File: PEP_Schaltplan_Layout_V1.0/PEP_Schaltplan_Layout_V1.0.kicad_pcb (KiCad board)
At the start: 2 copper layers, 117.5 x 83 mm, 120 parts, among them Q3 BC546, Q4 BC556, Q5 BF256, SW1 SW_DIP_x04, SW10 SW_DIP_x04, SW11 SW_DIP_x04, SW12 SW_DIP_x04, SW13 SW_DIP_x04, SW14 SW_DIP_x04, SW2 SW_DIP_x04, SW3 SW_DIP_x04, SW4 SW_DIP_x04, SW5 SW_DIP_x04, SW6 SW_DIP_x04, SW7 SW_DIP_x04, SW8 SW_DIP_x04, SW9 SW_DIP_x04, U12 AD822ANZ_new, U13 LT1819, U14 LT1819, U15 LT1819, U16 LT1819, U23 LM7905_TO220, U24 LM7805_TO220

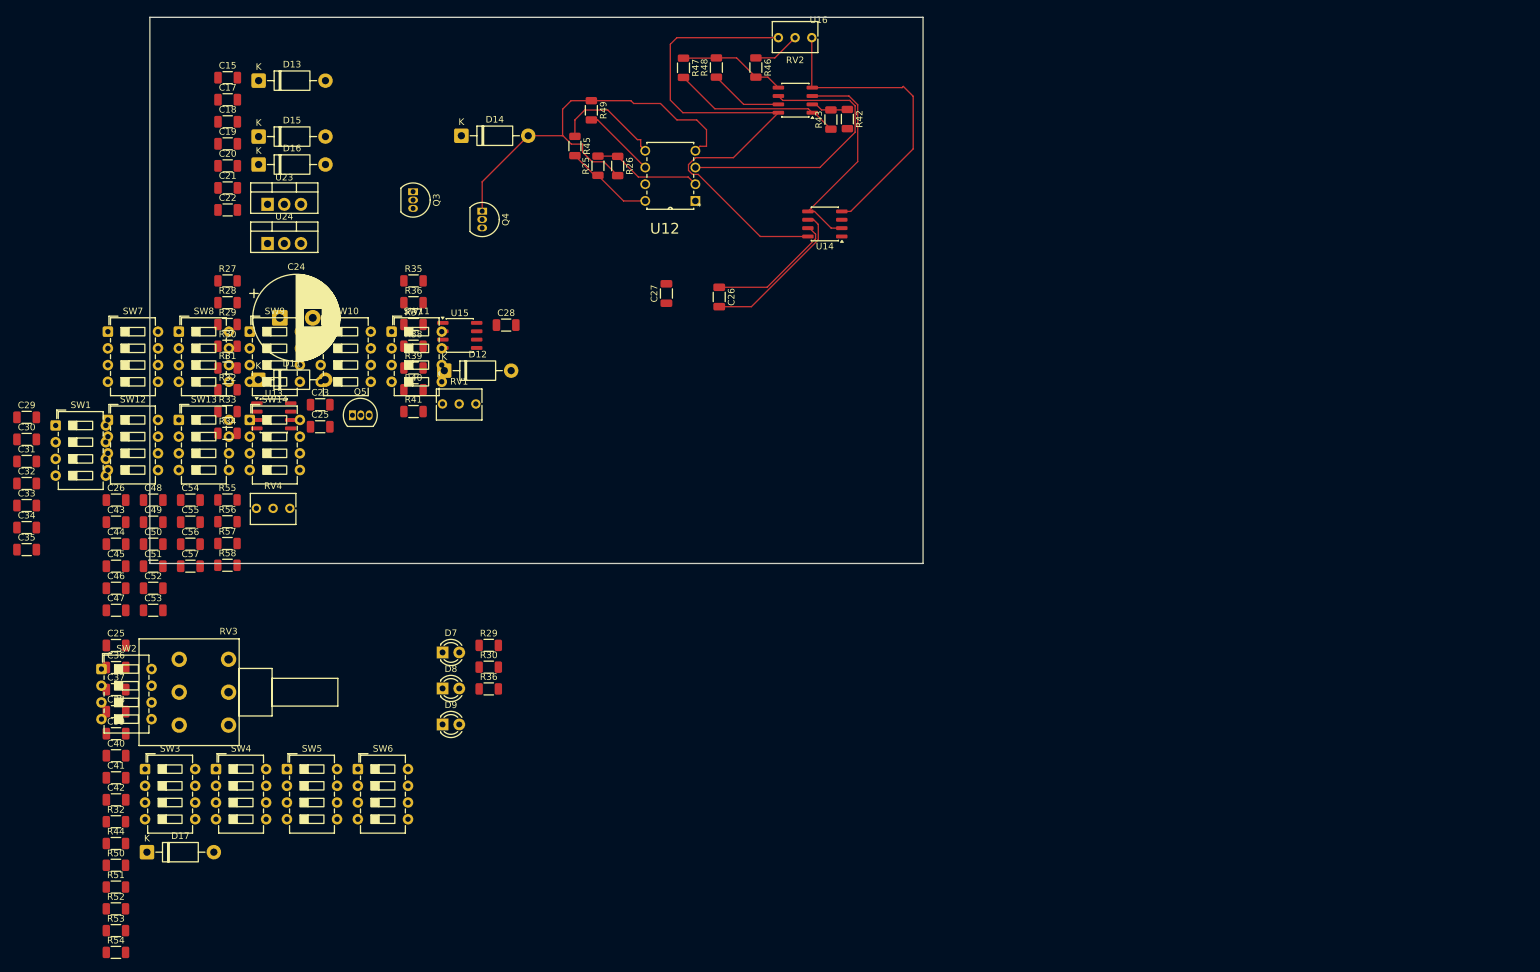
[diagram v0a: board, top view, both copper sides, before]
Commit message: Überarbeitung und Bereinigung
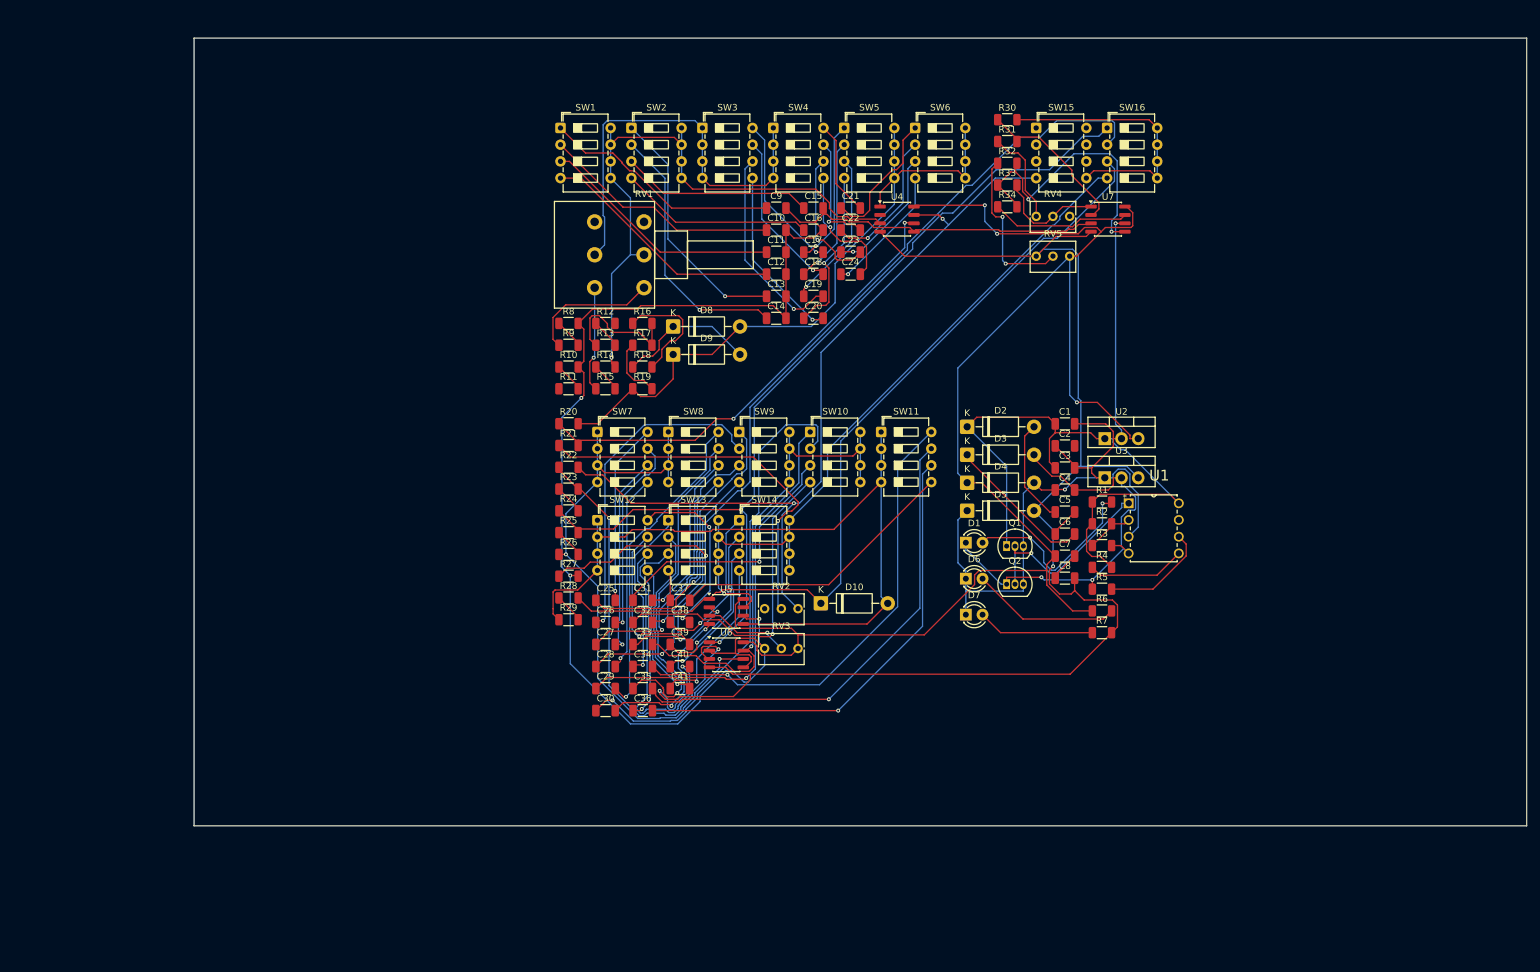
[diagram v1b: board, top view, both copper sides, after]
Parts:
- removed the C25 at (67.9, 99.7)
- removed the C25 at (36.9, 133.0)
- removed the C26 at (128.5, 80.0)
- removed the C26 at (36.9, 110.9)
- removed C42: 6.8n, Capacitor_SMD:C_1206_3216Metric
- removed C43, C50: 4.7n, Capacitor_SMD:C_1206_3216Metric
- removed C44: 470p, Capacitor_SMD:C_1206_3216Metric
- removed C45: 100p, Capacitor_SMD:C_1206_3216Metric
- removed C46, C53, C54: 47p, Capacitor_SMD:C_1206_3216Metric
- removed C47, C55: 22p, Capacitor_SMD:C_1206_3216Metric
- removed C48, C49, C56, C57: 0, Capacitor_SMD:C_1206_3216Metric
- removed C51: 1n, Capacitor_SMD:C_1206_3216Metric
- removed C52: 220p, Capacitor_SMD:C_1206_3216Metric
- removed D11, D12, D17: 1N4148, Diode_THT:D_DO-41_SOD81_P10.16mm_Horizontal
- removed D13, D14, D15, D16: 1N4002, Diode_THT:D_DO-41_SOD81_P10.16mm_Horizontal
- removed Q3: BC546, Package_TO_SOT_THT:TO-92_Inline
- removed Q4: BC556, Package_TO_SOT_THT:TO-92_Inline
- removed Q5: BF256, Package_TO_SOT_THT:TO-92L_Inline
- removed the R29 at (93.5, 132.9)
- removed the R29 at (53.8, 84.2)
- removed the R30 at (93.5, 136.3)
- removed the R30 at (53.8, 87.5)
- removed the R32 at (53.8, 94.1)
- removed the R32 at (36.8, 159.7)
- removed R35, R55: 1k, Resistor_SMD:R_1206_3216Metric
- removed R36: 2k2, Resistor_SMD:R_1206_3216Metric
- removed R36: 20k, Resistor_SMD:R_1206_3216Metric
- removed R37, R44, R46, R47, R48: 10k, Resistor_SMD:R_1206_3216Metric
- removed R38: 190k, Resistor_SMD:R_1206_3216Metric
- removed R39: 18k, Resistor_SMD:R_1206_3216Metric
- removed R40: 100k, Resistor_SMD:R_1206_3216Metric
- removed R41: 12k, Resistor_SMD:R_1206_3216Metric
- removed R42, R43: 5k, Resistor_SMD:R_1206_3216Metric
- removed R45, R49: R, Resistor_SMD:R_1206_3216Metric
- removed R50, R51, R52, R53, R54, R57, R58: 0, Resistor_SMD:R_1206_3216Metric
- removed R56: ^0, Resistor_SMD:R_1206_3216Metric
- removed U12: AD822ANZ_new, KiCad Footprint Bib:DIP8
- removed U13, U14, U15, U16: LT1819, Package_SO:SO-8_3.9x4.9mm_P1.27mm
- removed U23: LM7905_TO220, Package_TO_SOT_THT:TO-220-3_Vertical
- removed U24: LM7805_TO220, Package_TO_SOT_THT:TO-220-3_Vertical
- added C1: 1µ, Capacitor_SMD:C_1206_3216Metric, F.Cu at (181.1, 99.3)
- added C10: 6.8n, Capacitor_SMD:C_1206_3216Metric, F.Cu at (137.2, 69.8)
- added C11: 6.8n, Capacitor_SMD:C_1206_3216Metric, F.Cu at (137.2, 73.2)
- added C12: 6.8n, Capacitor_SMD:C_1206_3216Metric, F.Cu at (137.2, 76.5)
- added C13: 6.8n, Capacitor_SMD:C_1206_3216Metric, F.Cu at (137.2, 79.9)
- added C14: 6.8n, Capacitor_SMD:C_1206_3216Metric, F.Cu at (137.2, 83.2)
- added C16: 6.8n, Capacitor_SMD:C_1206_3216Metric, F.Cu at (142.8, 69.8)
- added C2: 1µ, Capacitor_SMD:C_1206_3216Metric, F.Cu at (181.1, 102.6)
- added C25: 22n, Capacitor_SMD:C_1206_3216Metric, F.Cu at (111.3, 126.1)
- added C26: 4.7n, Capacitor_SMD:C_1206_3216Metric, F.Cu at (111.3, 129.5)
- added C3: 100n, Capacitor_SMD:C_1206_3216Metric, F.Cu at (181.1, 106.0)
- added C4: 100n, Capacitor_SMD:C_1206_3216Metric, F.Cu at (181.1, 109.3)
- added C5: 1µ, Capacitor_SMD:C_1206_3216Metric, F.Cu at (181.1, 112.7)
- added C6: 1µ, Capacitor_SMD:C_1206_3216Metric, F.Cu at (181.1, 116.0)
- added C7: 100n, Capacitor_SMD:C_1206_3216Metric, F.Cu at (181.1, 119.4)
- added C8: 100n, Capacitor_SMD:C_1206_3216Metric, F.Cu at (181.1, 122.7)
- added C9: 6.8n, Capacitor_SMD:C_1206_3216Metric, F.Cu at (137.2, 66.5)
- added D1: LED, LED_THT:LED_D3.0mm, F.Cu at (166.0, 117.3)
- added D10: 1N4148, Diode_THT:D_DO-41_SOD81_P10.16mm_Horizontal, F.Cu at (144.0, 126.6)
- added D2: 1N4002, Diode_THT:D_DO-41_SOD81_P10.16mm_Horizontal, F.Cu at (166.2, 99.7)
- added D3: 1N4002, Diode_THT:D_DO-41_SOD81_P10.16mm_Horizontal, F.Cu at (166.2, 104.0)
- added D4: 1N4002, Diode_THT:D_DO-41_SOD81_P10.16mm_Horizontal, F.Cu at (166.2, 108.2)
- added D5: 1N4002, Diode_THT:D_DO-41_SOD81_P10.16mm_Horizontal, F.Cu at (166.2, 112.5)
- added D6: LED, LED_THT:LED_D3.0mm, F.Cu at (166.0, 122.8)
- added Q1: BC546, Package_TO_SOT_THT:TO-92_Inline, F.Cu at (172.2, 117.9)
- added Q2: BC556, Package_TO_SOT_THT:TO-92_Inline, F.Cu at (172.2, 123.7)
- added R1: 2k2, Resistor_SMD:R_1206_3216Metric, F.Cu at (186.7, 111.2)
- added R10: 0, Resistor_SMD:R_1206_3216Metric, F.Cu at (105.6, 90.6)
- added R11: 10k, Resistor_SMD:R_1206_3216Metric, F.Cu at (105.6, 94.0)
- added R12: 0, Resistor_SMD:R_1206_3216Metric, F.Cu at (111.2, 84.0)
- added R13: 10k, Resistor_SMD:R_1206_3216Metric, F.Cu at (111.2, 87.3)
- added R14: 500, Resistor_SMD:R_1206_3216Metric, F.Cu at (111.2, 90.6)
- added R15: 0, Resistor_SMD:R_1206_3216Metric, F.Cu at (111.2, 94.0)
- added R16: 24K, Resistor_SMD:R_1206_3216Metric, F.Cu at (116.8, 84.0)
- added R17: 12k, Resistor_SMD:R_1206_3216Metric, F.Cu at (116.8, 87.3)
- added R18: 0, Resistor_SMD:R_1206_3216Metric, F.Cu at (116.8, 90.6)
- added R19: 0, Resistor_SMD:R_1206_3216Metric, F.Cu at (116.8, 94.0)
- added R2: 47k, Resistor_SMD:R_1206_3216Metric, F.Cu at (186.7, 114.5)
- added R20: 1k, Resistor_SMD:R_1206_3216Metric, F.Cu at (105.6, 99.3)
- added R21: 1k, Resistor_SMD:R_1206_3216Metric, F.Cu at (105.6, 102.6)
- added R22: 10k, Resistor_SMD:R_1206_3216Metric, F.Cu at (105.6, 105.9)
- added R23: 190k, Resistor_SMD:R_1206_3216Metric, F.Cu at (105.6, 109.2)
- added R24: 0, Resistor_SMD:R_1206_3216Metric, F.Cu at (105.6, 112.5)
- added R29: ^0, Resistor_SMD:R_1206_3216Metric, F.Cu at (105.6, 129.1)
- added R3: 47k, Resistor_SMD:R_1206_3216Metric, F.Cu at (186.7, 117.8)
- added R30: 1k, Resistor_SMD:R_1206_3216Metric, F.Cu at (172.3, 53.1)
- added R32: 10k, Resistor_SMD:R_1206_3216Metric, F.Cu at (172.3, 59.7)
- added R4: R, Resistor_SMD:R_1206_3216Metric, F.Cu at (186.7, 121.1)
- added R5: R, Resistor_SMD:R_1206_3216Metric, F.Cu at (186.7, 124.4)
- added R6: 470, Resistor_SMD:R_1206_3216Metric, F.Cu at (186.7, 127.7)
- added R7: 470, Resistor_SMD:R_1206_3216Metric, F.Cu at (186.7, 131.0)
- added R8: 500, Resistor_SMD:R_1206_3216Metric, F.Cu at (105.6, 84.0)
- added R9: 0, Resistor_SMD:R_1206_3216Metric, F.Cu at (105.6, 87.3)
- added RV5: 10k, Potentiometer_THT:Potentiometer_Bourns_3266Y_Vertical, F.Cu at (181.8, 73.8)
- added SW15: SW_DIP_x04, Button_Switch_THT:SW_DIP_SPSTx04_Slide_6.7x11.72mm_W7.62mm_P2.54mm_LowProfile, F.Cu at (176.7, 54.3)
- added SW16: SW_DIP_x04, Button_Switch_THT:SW_DIP_SPSTx04_Slide_6.7x11.72mm_W7.62mm_P2.54mm_LowProfile, F.Cu at (187.5, 54.3)
- added U1: AD822ANZ_new, KiCad Footprint Bib:DIP8, F.Cu at (198.4, 119.0)
- added U2: LM7805_TO220, Package_TO_SOT_THT:TO-220-3_Vertical, F.Cu at (187.1, 101.5)
- added U3: LM7905_TO220, Package_TO_SOT_THT:TO-220-3_Vertical, F.Cu at (187.1, 107.5)
- added U4: LT1819, Package_SO:SO-8_3.9x4.9mm_P1.27mm, F.Cu at (155.5, 68.2)
- added U5: LT1819, Package_SO:SO-8_3.9x4.9mm_P1.27mm, F.Cu at (129.6, 127.8)
- added U6: LT1819, Package_SO:SO-8_3.9x4.9mm_P1.27mm, F.Cu at (129.6, 134.4)
- added U7: LT1819, Package_SO:SO-8_3.9x4.9mm_P1.27mm, F.Cu at (187.6, 68.2)
- C15, C19, C20: value 1µ -> 6.8n
- C17, C18, C21, C22: value 100n -> 6.8n
- C24: value 100µ -> 6.8n; footprint Capacitor_THT:CP_Radial_D13.0mm_P5.00mm -> Capacitor_SMD:C_1206_3216Metric
- C27: value 1µ -> 470p
- C28: value 4.7n -> 100p
- C29, C37, C38: value 6.8n -> 47p
- C30, C39: value 6.8n -> 22p
- C31, C32, C40, C41: value 6.8n -> 0
- C33: value 6.8n -> 1µ
- C34: value 6.8n -> 4.7n
- C35: value 6.8n -> 1n
- C36: value 6.8n -> 220p
- D8, D9: value LED -> 1N4148; footprint LED_THT:LED_D3.0mm -> Diode_THT:D_DO-41_SOD81_P10.16mm_Horizontal
- R25: value 47k -> 0
- R26: value 47k -> 18k
- R27: value 500 -> 100k
- R28: value 10k -> 12k
- R31: value 500 -> 1k
- R33: value 24K -> 10k
- R34: value 12k -> 10k
- RV1: value R_Potentiometer -> R_Potentiometer_Dual_Separate; footprint Potentiometer_THT:Potentiometer_Bourns_3266Y_Vertical -> Potentiometer_THT:Potentiometer_Piher_T-16H_Double_Horizontal
- RV2, RV4: value R_Potentiometer -> 10k
- RV3: value R_Potentiometer_Dual_Separate -> 10k; footprint Potentiometer_THT:Potentiometer_Piher_T-16H_Double_Horizontal -> Potentiometer_THT:Potentiometer_Bourns_3266Y_Vertical
- moved SW3 129.1 mm to (126.0, 54.3)
- moved SW4 129.1 mm to (136.7, 54.3)
- moved SW5 129.1 mm to (147.5, 54.3)
- moved SW6 129.1 mm to (158.3, 54.3)
- moved RV4 126.5 mm to (181.8, 67.8)
- moved R31 123.4 mm to (172.3, 56.4)
- moved R33 123.4 mm to (172.3, 63.0)
- moved R34 123.4 mm to (172.3, 66.3)
- moved SW2 115.1 mm to (115.2, 54.3)
- moved C29 97.2 mm to (111.3, 139.5)
- moved C30 97.2 mm to (111.3, 142.9)
- moved C31 96.0 mm to (116.9, 126.1)
- moved C33 96.0 mm to (116.9, 132.8)
- moved C34 96.0 mm to (116.9, 136.2)
- moved C35 96.0 mm to (116.9, 139.5)
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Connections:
- C15 pad 1: +7.5V -> Net-(C15-Pad1)
- C15 pad 2: GND -> 0
- C17 pad 1: +7.5V -> Net-(C17-Pad1)
- C17 pad 2: GND -> Net-(C17-Pad2)
- C18 pad 1: GND -> Net-(C18-Pad1)
- C18 pad 2: unconnected-(C18-Pad2) -> Net-(C18-Pad2)
- C19 pad 1: Net-(D13-A) -> Net-(C19-Pad1)
- C20 pad 1: Net-(C19-Pad2) -> Net-(C20-Pad1)
- C20 pad 2: Net-(D14-K) -> Net-(C20-Pad2)
- C21 pad 1: +5V -> Net-(C21-Pad1)
- C22 pad 1: Net-(C21-Pad2) -> Net-(C22-Pad1)
- C22 pad 2: -5V -> Net-(C22-Pad2)
- C23 pad 2: 0 -> Net-(C23-Pad2)
- C24 pad 1: Net-(D11-+) -> Net-(C24-Pad1)
- C24 pad 2: 0 -> Net-(C24-Pad2)
- C27 pad 1: Dreieck -> Net-(C27-Pad1)
- C28 pad 1: Sägezahn -> Net-(C28-Pad1)
- C28 pad 2: Net-(D12--) -> Net-(C28-Pad2)
- C29 pad 2: 0 -> Net-(C29-Pad2)
- C30 pad 2: 0 -> Net-(C30-Pad2)
- C31 pad 2: 0 -> Net-(C31-Pad2)
- C32 pad 2: 0 -> Net-(C32-Pad2)
- C33 pad 1: Net-(C33-Pad1) -> Dreieck
- C33 pad 2: 0 -> Net-(C33-Pad2)
- C34 pad 2: 0 -> Net-(C34-Pad2)
- C35 pad 2: 0 -> Net-(C35-Pad2)
- D8 pad 1: GND -> Net-(D8-+)
- D8 pad 2: Net-(D8-A) -> Sinus_Wien
- D9 pad 1: -7.5V -> Sinus_Wien
- D9 pad 2: Net-(D9-A) -> Net-(D8-+)
- R25 pad 1: +7.5V -> Net-(R25-Pad1)
- R25 pad 2: Net-(U12A--) -> Rechteck
- R26 pad 1: Net-(U12A--) -> Net-(U6B--)
- R26 pad 2: -7.5V -> Net-(R25-Pad1)
- R27 pad 1: Net-(R27-Pad1) -> Dreieck
- R28 pad 2: Net-(R28-Pad2) -> PWM
- R31 pad 2: Net-(U13A-+) -> Net-(U7A--)
- R33 pad 1: Net-(R33-Pad1) -> Net-(U7B-+)
- R34 pad 1: Net-(R34-Pad1) -> offset
- R34 pad 2: Net-(R33-Pad2) -> Net-(U7B-+)
- RV1 pad 1: +5v -> Net-(R9-Pad1)
- RV1 pad 2: Net-(U15A-+) -> Net-(U4A-+)
- RV1 pad 3: 0 -> unconnected-(RV1-Pad3)
- RV2 pad 1: +5v -> Sinus
- RV2 pad 3: -5v -> unconnected-(RV2-Pad3)
- RV3 pad 1: Net-(R50-Pad1) -> +5V
- RV3 pad 2: Net-(U13A-+) -> Net-(U5A-+)
- RV3 pad 3: unconnected-(RV3-Pad3) -> 0
- RV4 pad 1: Sinus -> unconnected-(RV4-Pad1)
- RV4 pad 2: Net-(R55-Pad1) -> Net-(R33-Pad2)
- RV4 pad 3: unconnected-(RV4-Pad3) -> Net-(R31-Pad1)
- SW1 pad 1: Net-(C23-Pad1) -> Net-(C9-Pad1)
- SW1 pad 2: Net-(C29-Pad1) -> Net-(C10-Pad1)
- SW1 pad 3: Net-(C30-Pad1) -> Net-(C11-Pad1)
- SW1 pad 4: Net-(C31-Pad1) -> Net-(C12-Pad1)
- SW1 pad 5: Net-(U13A-+) -> Net-(U4A-+)
- SW1 pad 6: Net-(U13A-+) -> Net-(U4A-+)
- SW1 pad 7: Net-(U13A-+) -> Net-(U4A-+)
- SW1 pad 8: Net-(U13A-+) -> Net-(U4A-+)
- SW10 pad 1: Net-(C46-Pad1) -> Net-(C29-Pad1)
- SW10 pad 2: Net-(C47-Pad1) -> Net-(C30-Pad1)
- SW10 pad 3: Net-(C48-Pad1) -> Net-(C31-Pad1)
- SW10 pad 4: Net-(C49-Pad1) -> Net-(C32-Pad1)
- SW10 pad 5: Net-(C27-Pad2) -> Net-(C33-Pad2)
- SW10 pad 6: Net-(C27-Pad2) -> Net-(C33-Pad2)
- SW10 pad 7: Net-(C27-Pad2) -> Net-(C33-Pad2)
- SW10 pad 8: Net-(C27-Pad2) -> Net-(C33-Pad2)
- SW11 pad 1: Net-(D12--) -> Net-(D10--)
- SW11 pad 2: Net-(D12--) -> Net-(D10--)
- SW11 pad 3: Net-(D12--) -> Net-(D10--)
- SW11 pad 4: Net-(D12--) -> Net-(D10--)
- SW11 pad 5: Net-(C53-Pad2) -> Net-(C37-Pad2)
- SW11 pad 6: Net-(C52-Pad2) -> Net-(C36-Pad2)
- SW11 pad 7: Net-(C51-Pad2) -> Net-(C35-Pad2)
- SW11 pad 8: Net-(C50-Pad2) -> Net-(C34-Pad2)
- SW12 pad 1: Net-(D12--) -> Net-(D10--)
- SW12 pad 2: Net-(D12--) -> Net-(D10--)
- SW12 pad 3: Net-(D12--) -> Net-(D10--)
- SW12 pad 4: Net-(D12--) -> Net-(D10--)
- SW12 pad 5: Net-(C57-Pad2) -> Net-(C41-Pad2)
- SW12 pad 6: Net-(C56-Pad2) -> Net-(C40-Pad2)
- SW12 pad 7: Net-(C55-Pad2) -> Net-(C39-Pad2)
- SW12 pad 8: Net-(C54-Pad2) -> Net-(C38-Pad2)
- SW13 pad 1: Net-(C50-Pad1) -> Net-(C34-Pad1)
- SW13 pad 2: Net-(C51-Pad1) -> Net-(C35-Pad1)
- SW13 pad 3: Net-(C52-Pad1) -> Net-(C36-Pad1)
- SW13 pad 4: Net-(C53-Pad1) -> Net-(C37-Pad1)
- SW14 pad 1: Net-(C54-Pad1) -> Net-(C38-Pad1)
- SW14 pad 2: Net-(C55-Pad1) -> Net-(C39-Pad1)
- SW14 pad 3: Net-(C56-Pad1) -> Net-(C40-Pad1)
- SW14 pad 4: Net-(C57-Pad1) -> Net-(C41-Pad1)
- SW2 pad 1: Net-(C32-Pad1) -> Net-(C13-Pad1)
- SW2 pad 2: Net-(C33-Pad1) -> Net-(C14-Pad1)
- SW2 pad 3: Net-(C34-Pad1) -> Net-(C15-Pad1)
- SW2 pad 4: Net-(C35-Pad1) -> Net-(C16-Pad1)
- SW2 pad 5: Net-(U13A-+) -> Net-(U4A-+)
- SW2 pad 6: Net-(U13A-+) -> Net-(U4A-+)
- SW2 pad 7: Net-(U13A-+) -> Net-(U4A-+)
- SW2 pad 8: Net-(U13A-+) -> Net-(U4A-+)
- SW3 pad 1: Net-(C25-Pad1) (its old number) -> Net-(RV1-Pad5)
- SW3 pad 2: Net-(C36-Pad1) -> Net-(RV1-Pad5)
- SW3 pad 3: Net-(C37-Pad1) -> Net-(RV1-Pad5)
- SW3 pad 4: Net-(C38-Pad1) -> Net-(RV1-Pad5)
- SW3 pad 5: /Wien-Robinson-Generator/Sinus -> Net-(C20-Pad2)
- SW3 pad 6: /Wien-Robinson-Generator/Sinus -> Net-(C19-Pad2)
- SW3 pad 7: /Wien-Robinson-Generator/Sinus -> Net-(C18-Pad2)
- SW3 pad 8: /Wien-Robinson-Generator/Sinus -> Net-(C17-Pad2)
- SW4 pad 1: Net-(C39-Pad1) -> Net-(RV1-Pad5)
- SW4 pad 2: Net-(C40-Pad1) -> Net-(RV1-Pad5)
- SW4 pad 3: Net-(C41-Pad1) -> Net-(RV1-Pad5)
- SW4 pad 4: Net-(C42-Pad1) -> Net-(RV1-Pad5)
- SW4 pad 5: /Wien-Robinson-Generator/Sinus -> Net-(C24-Pad2)
- SW4 pad 6: /Wien-Robinson-Generator/Sinus -> Net-(C23-Pad2)
- SW4 pad 7: /Wien-Robinson-Generator/Sinus -> Net-(C22-Pad2)
- SW4 pad 8: /Wien-Robinson-Generator/Sinus -> Net-(C21-Pad2)
- SW5 pad 1: Net-(RV3-Pad5) -> Net-(C17-Pad1)
- SW5 pad 2: Net-(RV3-Pad5) -> Net-(C18-Pad1)
- SW5 pad 3: Net-(RV3-Pad5) -> Net-(C19-Pad1)
- SW5 pad 4: Net-(RV3-Pad5) -> Net-(C20-Pad1)
- SW5 pad 5: Net-(C38-Pad2) -> Sinus_Wien
- SW5 pad 6: Net-(C37-Pad2) -> Sinus_Wien
- SW5 pad 7: Net-(C36-Pad2) -> Sinus_Wien
- SW5 pad 8: Net-(C25-Pad2) (its old number) -> Sinus_Wien
- SW6 pad 1: Net-(RV3-Pad5) -> Net-(C21-Pad1)
- SW6 pad 2: Net-(RV3-Pad5) -> Net-(C22-Pad1)
- SW6 pad 3: Net-(RV3-Pad5) -> Net-(C23-Pad1)
- SW6 pad 4: Net-(RV3-Pad5) -> Net-(C24-Pad1)
- SW6 pad 5: Net-(C42-Pad2) -> Sinus_Wien
- SW6 pad 6: Net-(C41-Pad2) -> Sinus_Wien
- SW6 pad 7: Net-(C40-Pad2) -> Sinus_Wien
- SW6 pad 8: Net-(C39-Pad2) -> Sinus_Wien
- SW7 pad 1: Net-(U14B--) -> Net-(U6B--)
- SW7 pad 2: Net-(U14B--) -> Net-(U6B--)
- SW7 pad 3: Net-(U14B--) -> Net-(U6B--)
- SW7 pad 4: Net-(U14B--) -> Net-(U6B--)
- SW7 pad 5: Net-(C45-Pad2) -> Net-(C28-Pad2)
- SW7 pad 6: Net-(C44-Pad2) -> Net-(C27-Pad2)
- SW8 pad 1: Net-(U14B--) -> Net-(U6B--)
- SW8 pad 2: Net-(U14B--) -> Net-(U6B--)
- SW8 pad 3: Net-(U14B--) -> Net-(U6B--)
- SW8 pad 4: Net-(U14B--) -> Net-(U6B--)
- SW8 pad 5: Net-(C49-Pad2) -> Net-(C32-Pad2)
- SW8 pad 6: Net-(C48-Pad2) -> Net-(C31-Pad2)
- SW8 pad 7: Net-(C47-Pad2) -> Net-(C30-Pad2)
- SW8 pad 8: Net-(C46-Pad2) -> Net-(C29-Pad2)
- SW9 pad 3: Net-(C44-Pad1) -> Net-(C27-Pad1)
- SW9 pad 4: Net-(C45-Pad1) -> Net-(C28-Pad1)
- SW9 pad 5: Net-(C27-Pad2) -> Net-(C33-Pad2)
- SW9 pad 6: Net-(C27-Pad2) -> Net-(C33-Pad2)
- SW9 pad 7: Net-(C27-Pad2) -> Net-(C33-Pad2)
- SW9 pad 8: Net-(C27-Pad2) -> Net-(C33-Pad2)
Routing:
- net -5V: track 0.00 -> 226.5 mm, vias 0 -> 3
- net +5V: track 0.00 -> 225.2 mm, vias 0 -> 3
- net 0: track 33.0 -> 227.0 mm, vias 0 -> 3
- net Dreieck: track 0.00 -> 159.9 mm, vias 0 -> 3
- net Rechteck: track 0.00 -> 142.4 mm, vias 0 -> 2
- net Sinus: track 0.00 -> 127.5 mm, vias 0 -> 2
- net PWM: track 0.00 -> 127.3 mm
- net Net-(D10--): track 0.00 -> 116.8 mm
- net Sägezahn: track 0.00 -> 110.3 mm, vias 0 -> 1
- net Sinus_Wien: track 0.00 -> 104.7 mm
- net Net-(U4A-+): track 0.00 -> 93.9 mm, vias 0 -> 1
- net Net-(U6B--): track 0.00 -> 91.6 mm, vias 0 -> 2
- net GND: track 42.8 -> 129.6 mm, vias 0 -> 2
- net +5v: track 82.7 -> 0.00 mm
- net +7.5V: track 13.5 -> 92.8 mm
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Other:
- board size 117.5 x 83 mm -> 202.5 x 119.7 mm
